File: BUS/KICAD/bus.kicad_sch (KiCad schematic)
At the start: 8 parts

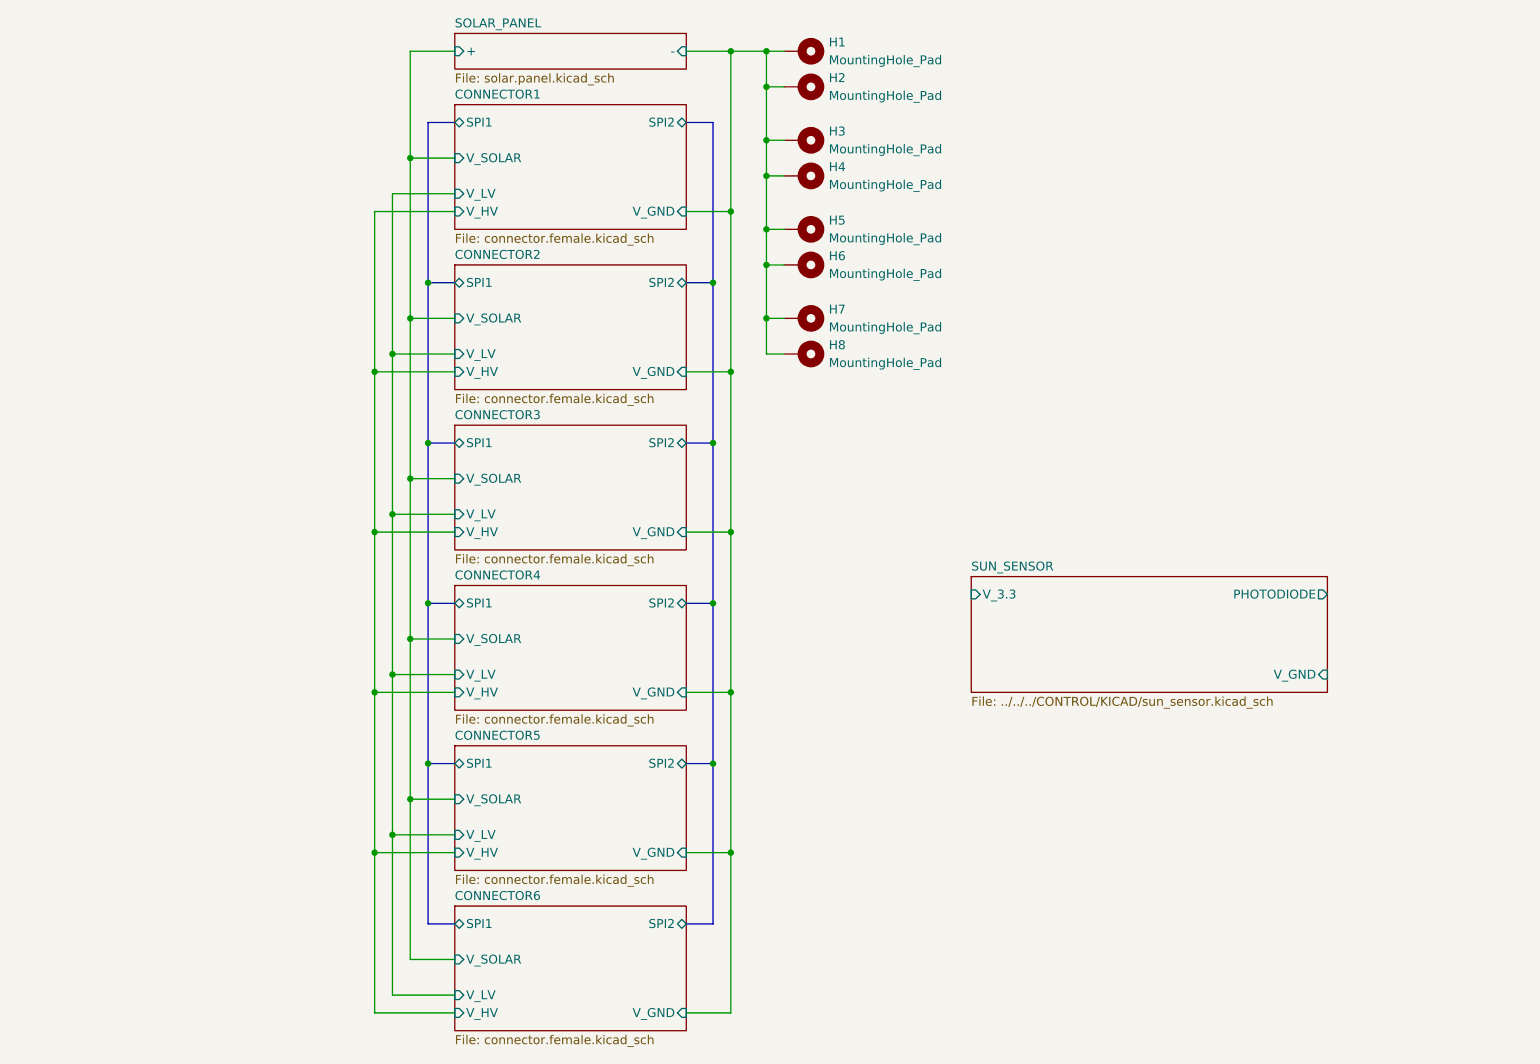
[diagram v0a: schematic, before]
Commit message: Updated Bus
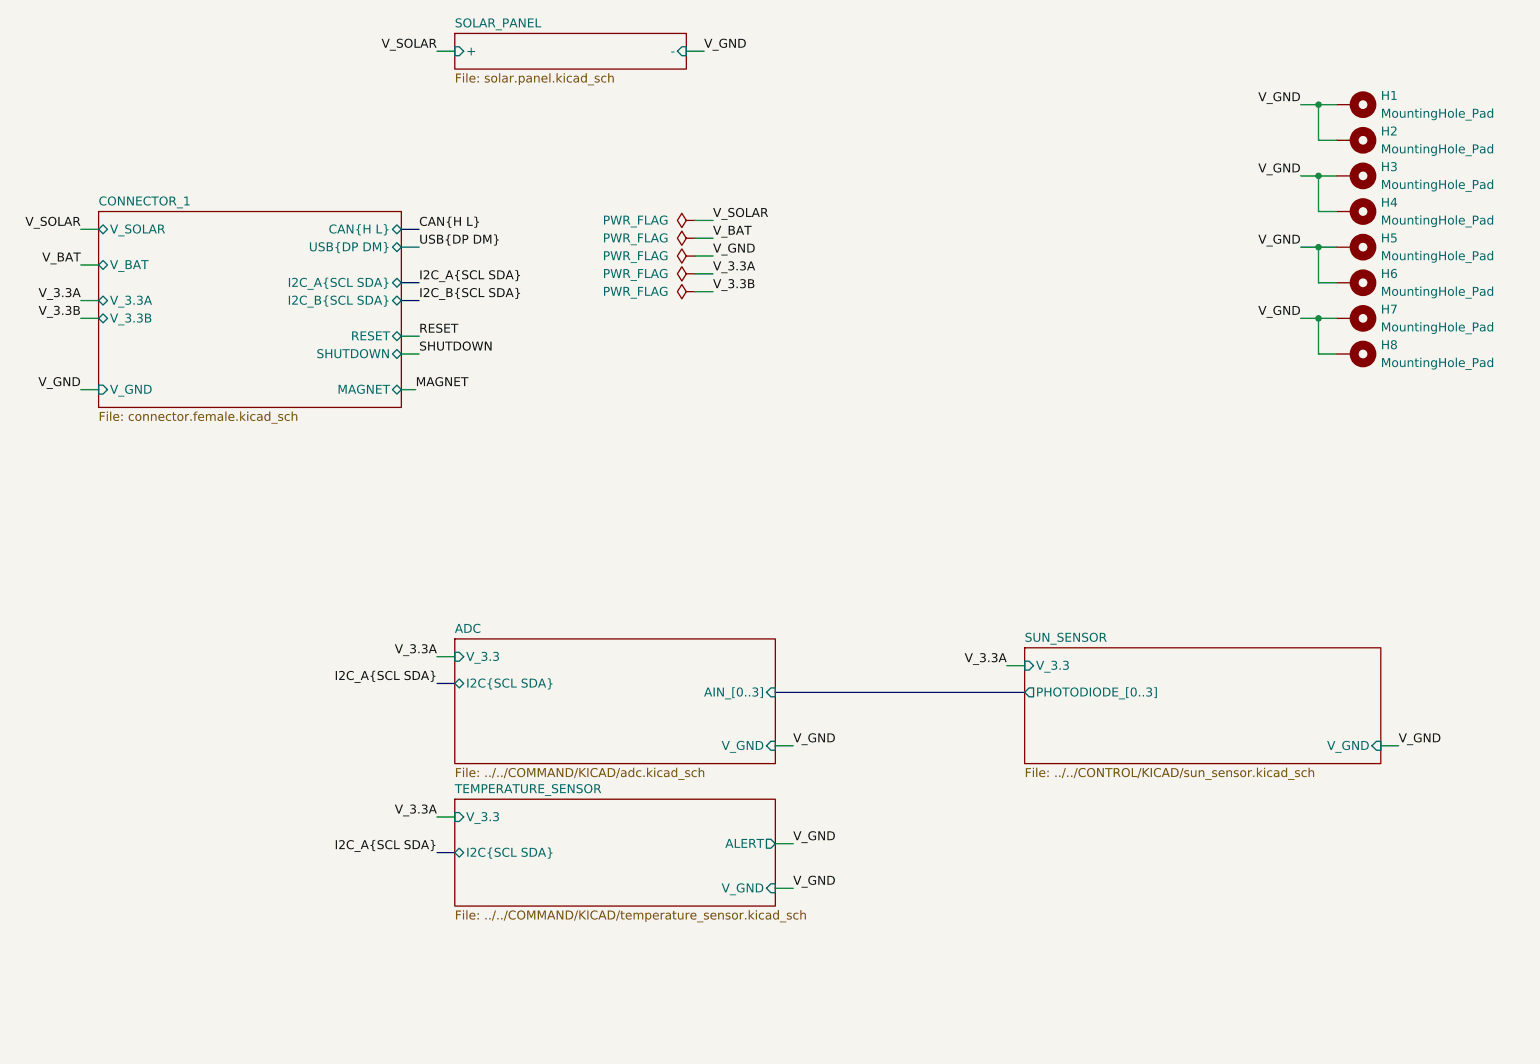
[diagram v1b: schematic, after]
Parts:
- H1, H2, H3, H4, H5, H6, H7, H8: footprint (none) -> MountingHole:MountingHole_3.2mm_M3_Pad_TopBottom
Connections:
- net CONNECTOR1/V_GND renamed V_GND
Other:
- removed sheet CONNECTOR1
- removed sheet CONNECTOR2
- removed sheet CONNECTOR3
- removed sheet CONNECTOR4
- removed sheet CONNECTOR5
- removed sheet CONNECTOR6
- added sheet ADC (../../COMMAND/KICAD/adc.kicad_sch)
- added sheet CONNECTOR_1 (connector.female.kicad_sch)
- added sheet TEMPERATURE_SENSOR (../../COMMAND/KICAD/temperature_sensor.kicad_sch)
- sheet SUN_SENSOR: file ../../../CONTROL/KICAD/sun_sensor.kicad_sch -> ../../CONTROL/KICAD/sun_sensor.kicad_sch
- sheet SUN_SENSOR ports: added PHOTODIODE_[0..3]; removed PHOTODIODE
- moved on the sheet: H7, H8
